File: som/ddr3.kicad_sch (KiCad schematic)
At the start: 6 parts, among them U2 AS4C256M16D3, U3 AS4C256M16D3

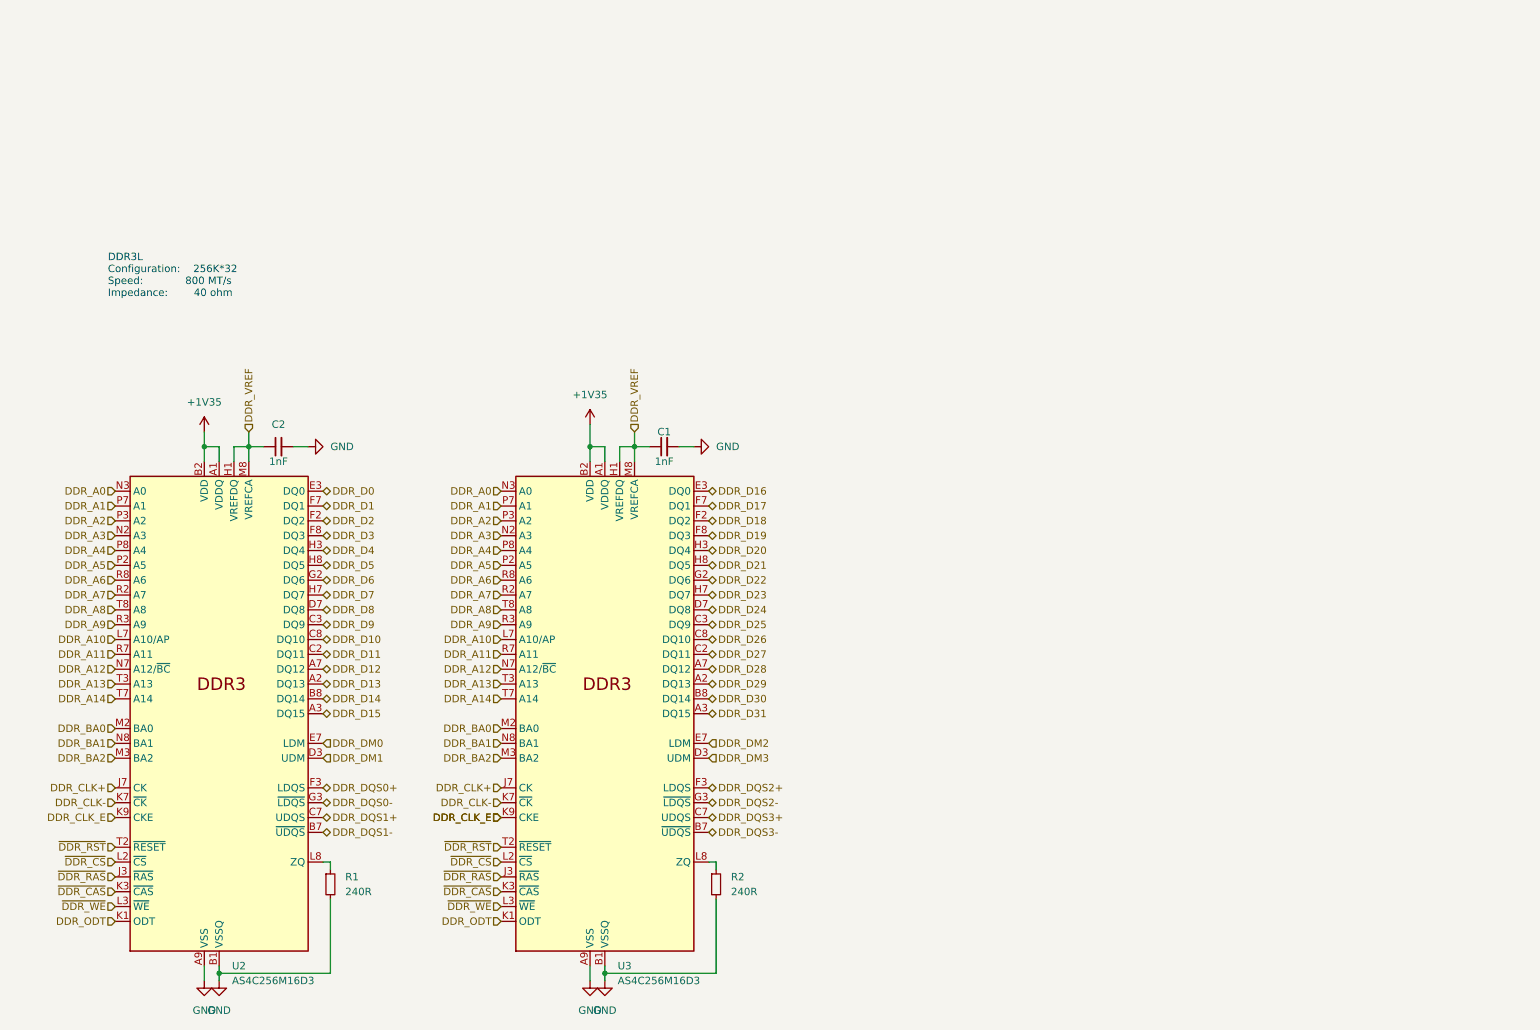
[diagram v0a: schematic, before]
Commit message: ok
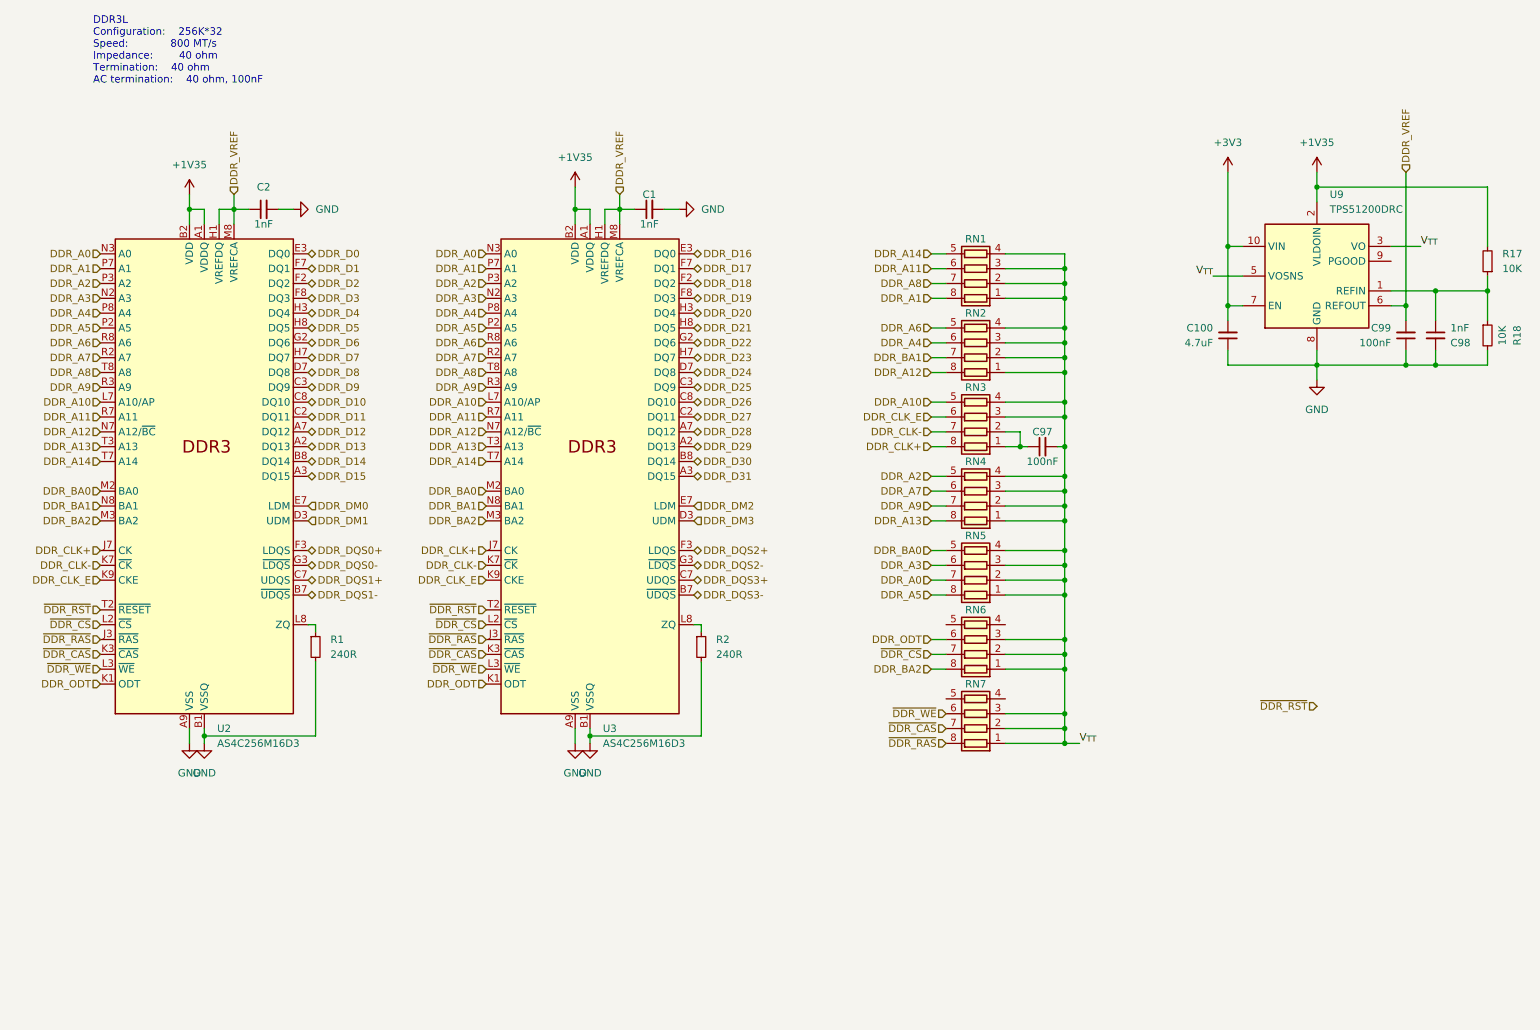
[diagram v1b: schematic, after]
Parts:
- added C100: 4.7uF, Capacitor_SMD:C_0402_1005Metric, symbol Device:C_Small
- added C97, C99: 100nF, Capacitor_SMD:C_0402_1005Metric, symbol Device:C_Small
- added C98: 1nF, Capacitor_SMD:C_0402_1005Metric, symbol Device:C_Small
- added R17, R18: 10K, Resistor_SMD:R_0402_1005Metric_Pad0.72x0.64mm_HandSolder, symbol Device:R_Small
- added RN1, RN2, RN3, RN4, RN5, RN6, RN7: R_Pack04, Resistor_SMD:R_Array_Concave_4x0402, symbol Device:R_Pack04
- added U9: TPS51200DRC, Package_SON:VSON-10-1EP_3x3mm_P0.5mm_EP1.65x2.4mm, symbol Regulator_Linear:TPS51200DRC
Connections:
- net +1V35: now also R17.2, U9.2 (VLDOIN)
- net DDR_A0: now also RN5.7 (R2.2)
- net DDR_A1: now also RN1.8 (R1.2)
- net DDR_A10: now also RN3.5 (R4.2)
- net DDR_A11: now also RN1.6 (R3.2)
- net DDR_A12: now also RN2.8 (R1.2)
- net DDR_A13: now also RN4.8 (R1.2)
- net DDR_A14: now also RN1.5 (R4.2)
- net DDR_A2: now also RN4.5 (R4.2)
- net DDR_A3: now also RN5.6 (R3.2)
- net DDR_A4: now also RN2.6 (R3.2)
- net DDR_A5: now also RN5.8 (R1.2)
- net DDR_A6: now also RN2.5 (R4.2)
- net DDR_A7: now also RN4.6 (R3.2)
- net DDR_A8: now also RN1.7 (R2.2)
- net DDR_A9: now also RN4.7 (R2.2)
- net DDR_BA0: now also RN5.5 (R4.2)
- net DDR_BA1: now also RN2.7 (R2.2)
- net DDR_BA2: now also RN6.8 (R1.2)
- net DDR_CLK+: now also RN3.8 (R1.2)
- net DDR_CLK-: now also RN3.7 (R2.2)
- net DDR_CLK_E: now also RN3.6 (R3.2)
- net DDR_ODT: now also RN6.6 (R3.2)
- net DDR_VREF: now also C99.2, U9.6 (REFOUT)
- net GND: now also C100.1, C98.2, C99.1, R18.2, U9.11 (GND), U9.4 (GND), U9.8 (GND)
- net ~{DDR_CAS}: now also RN7.7 (R2.2)
- net ~{DDR_CS}: now also RN6.7 (R2.2)
- net ~{DDR_RAS}: now also RN7.8 (R1.2)
- net ~{DDR_WE}: now also RN7.6 (R3.2)
- new net: C98.1, R17.1, R18.1, U9.1 (REFIN)
- new net: C97.1, RN3.1 (R1.1), RN3.2 (R2.1)
- new net +3V3: C100.2, U9.10 (VIN), U9.7 (EN)
- new net V_{TT}: C97.2, RN1.1 (R1.1), RN1.2 (R2.1), RN1.3 (R3.1), RN1.4 (R4.1), RN2.1 (R1.1), RN2.2 (R2.1), RN2.3 (R3.1), RN2.4 (R4.1), RN3.3 (R3.1), RN3.4 (R4.1), RN4.1 (R1.1), RN4.2 (R2.1), RN4.3 (R3.1), RN4.4 (R4.1), RN5.1 (R1.1), RN5.2 (R2.1), RN5.3 (R3.1), RN5.4 (R4.1), RN6.1 (R1.1), RN6.2 (R2.1), RN6.3 (R3.1), RN7.1 (R1.1), RN7.2 (R2.1), RN7.3 (R3.1), U9.3 (VO), U9.5 (VOSNS)
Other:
- note added: "DDR3L Configuration: 256K*32 Speed: 800 MT/s Impedance: 40 ohm Termination: 40 ohm AC termination: 40 ohm, 100nF"
- note removed: "DDR3L Configuration: 256K*32 Speed: 800 MT/s Impedance: 40 ohm"
- moved on the sheet: C1, C2, R1, R2, U2, U3
